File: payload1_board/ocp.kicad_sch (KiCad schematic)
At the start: 22 parts, among them Q2 SSM6K403TU_LF, U6 LTC4361HTS8-2-TRMPBF

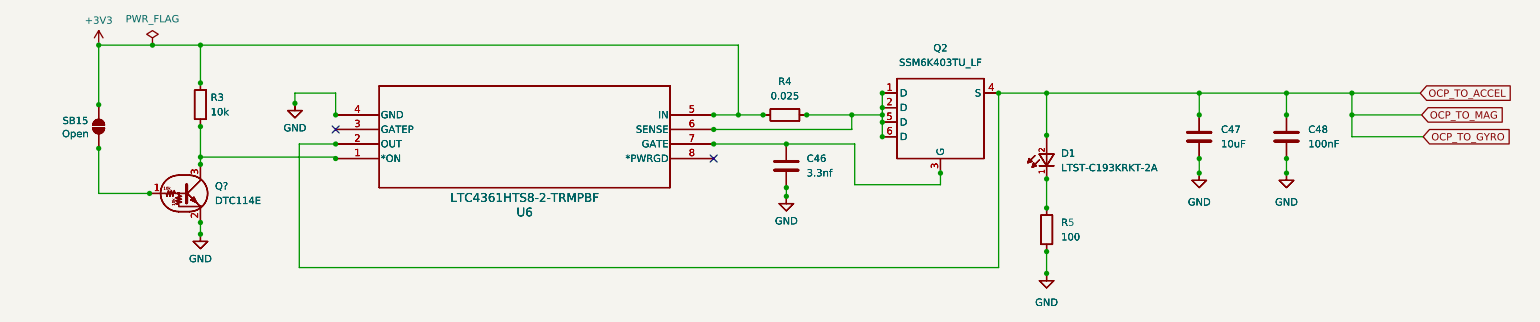
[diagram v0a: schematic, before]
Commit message: 1st debugging
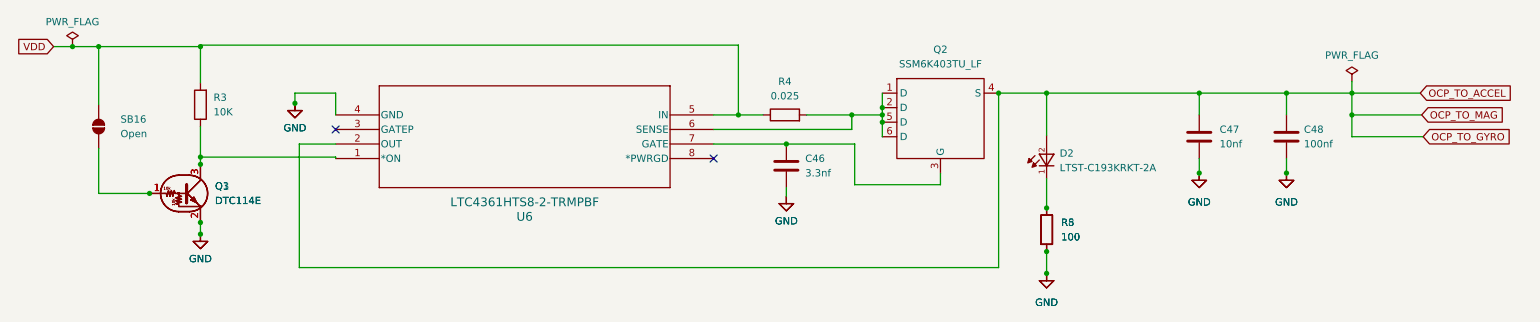
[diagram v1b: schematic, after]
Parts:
- removed C46 (x2): 3.3nf, symbol Device:C
- removed C47 (x2): 10uF, Capacitor_SMD:C_0805_2012Metric, symbol Device:C
- removed C48 (x2): 100nF, Capacitor_SMD:C_0805_2012Metric, symbol Device:C
- removed D1 (x2): LTST-C193KRKT-2A, LTST-C193KRKT-2A:0603, symbol LTST-C193KRKT-2A:LTST-C193KRKT-2A
- removed Q2 (x2): SSM6K403TU_LF, SSM6K403TU_LF:UF6_TOS-L, symbol SSM6K403TU_LF:SSM6K403TU_LF
- removed R3 (x2): 10k, symbol Device:R
- removed R4 (x2): 0.025, symbol Device:R
- removed SB15 (x2): Open, symbol Jumper:SolderJumper_2_Open
- removed U6 (x2): LTC4361HTS8-2-TRMPBF, TSOT-23_TS8_LIT, symbol 2024-08-14_17-14-28:LTC4361HTS8-2-TRMPBF
- added C46: 3.3nf, symbol Device:C
- added C47: 10nf, symbol Device:C
- added C48: 100nf, symbol Device:C
- added D2: LTST-C193KRKT-2A, LTST-C193KRKT-2A:0603, symbol LTST-C193KRKT-2A:LTST-C193KRKT-2A
- added Q2: SSM6K403TU_LF, SSM6K403TU_LF:UF6_TOS-L, symbol SSM6K403TU_LF:SSM6K403TU_LF
- added R3: 10K, symbol Device:R
- added R4: 0.025, symbol Device:R
- added SB16: Open, symbol Jumper:SolderJumper_2_Open
- added U6: LTC4361HTS8-2-TRMPBF, TSOT-23_TS8_LIT, symbol 2024-08-14_17-14-28:LTC4361HTS8-2-TRMPBF
- gave numbers to parts that had none: 2
- renumbered R to R8
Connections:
- net GND: now also C46.2, C47.2, C48.2, U6.4 (GND)
- net OCP_TO_ACCEL: now also C47.1, C48.1, D2.2, Q2.4 (S), U6.2 (OUT)
- net at Q1.1 (B), Q3.1 (B): now also SB16.1 (A)
- net at Q1.3 (C), Q3.3 (C): now also R3.1, U6.1 (*ON)
- net at R5.2, R8.2: now also D2.1
- new net: C46.1, Q2.3 (G), U6.7 (GATE)
- new net: Q2.1 (D), Q2.2 (D), Q2.5 (D), Q2.6 (D), R4.2, U6.6 (SENSE)
- new net VDD: R3.2, R4.1, SB16.2 (B), U6.5 (IN)
